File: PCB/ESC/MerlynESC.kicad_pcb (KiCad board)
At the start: 4 copper layers, 30.5 x 31.9 mm, 155 parts, among them M1 BLDC Motor, M2 BLDC Motor, M3 BLDC Motor, M4 BLDC Motor, Q1 JMSL0302AU, Q10 JMSL0302AU, Q11 JMSL0302AU, Q12 JMSL0302AU, Q13 JMSL0302AU, Q14 JMSL0302AU, Q15 JMSL0302AU, Q16 JMSL0302AU, Q17 JMSL0302AU, Q18 JMSL0302AU, Q19 JMSL0302AU, Q2 JMSL0302AU, Q20 JMSL0302AU, Q21 JMSL0302AU, Q22 JMSL0302AU, Q23 JMSL0302AU, Q24 JMSL0302AU, Q3 JMSL0302AU, Q4 JMSL0302AU, Q5 JMSL0302AU, Q6 JMSL0302AU, Q7 JMSL0302AU, Q8 JMSL0302AU, Q9 JMSL0302AU, U1 HT75C0-1, U10 EG6288, U11 EFM8BB21F16G, U2 HT7533-1, U3 EFM8BB21F16G, U4 EG6288, U5 EG6288, U6 EFM8BB21F16G, U7 INA139NA, U8 EG6288, U9 EFM8BB21F16G

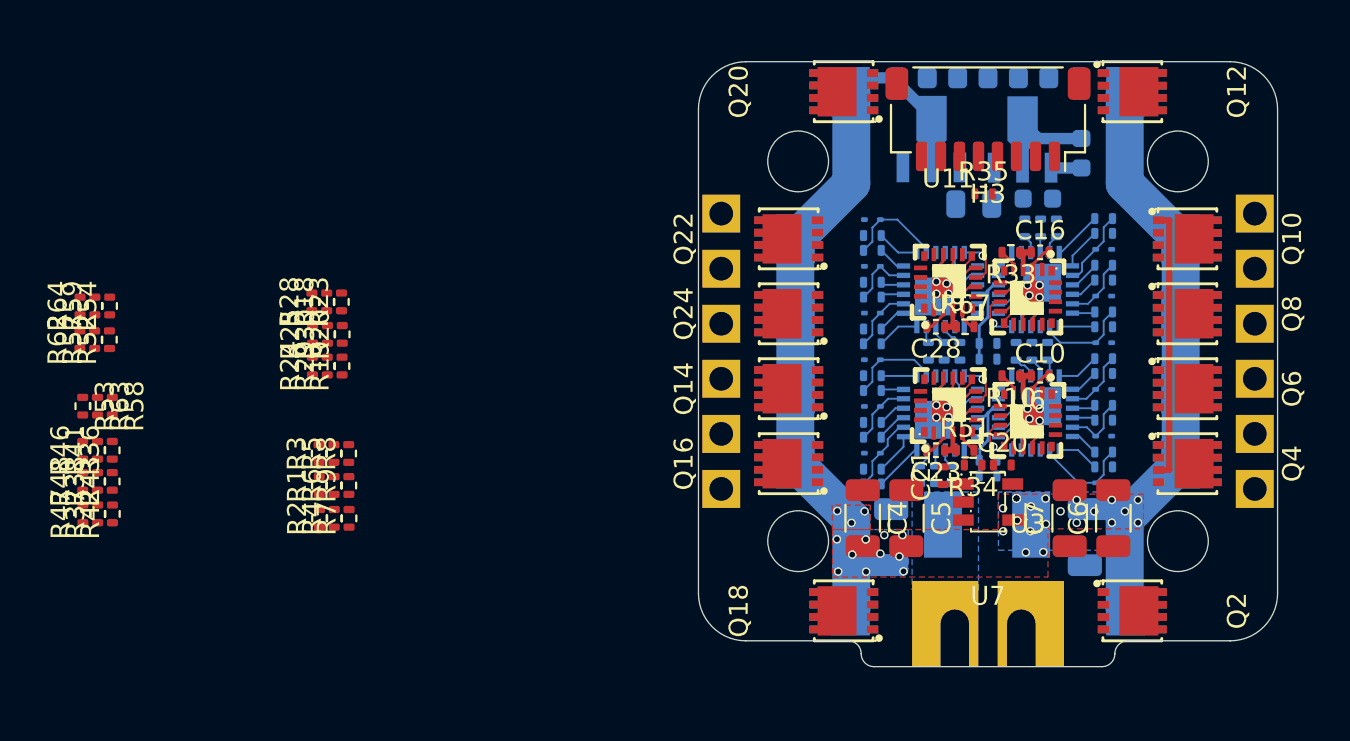
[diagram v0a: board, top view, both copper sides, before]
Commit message: checkpoint
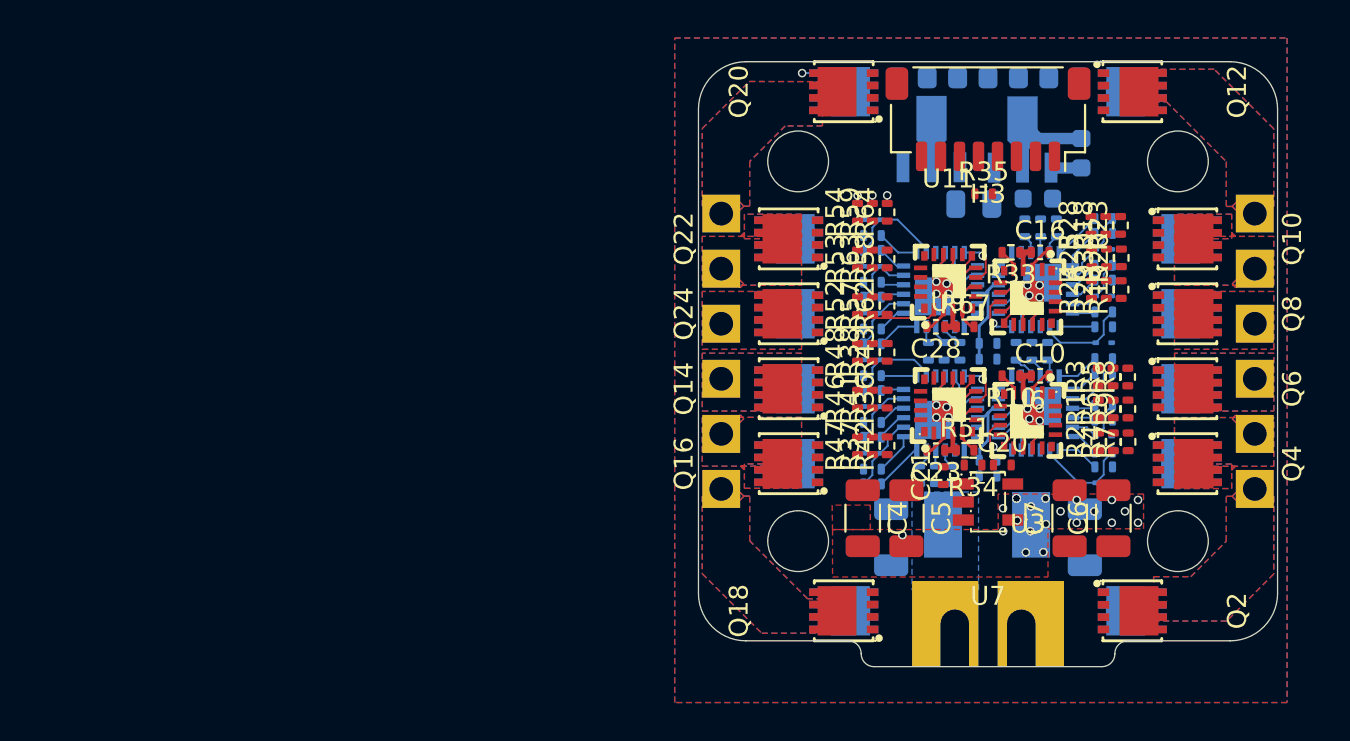
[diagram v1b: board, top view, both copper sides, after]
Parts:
- moved R64 42.8 mm to (150.1, 94.6)
- moved R62 42.6 mm to (150.1, 99.5)
- moved R53 41.5 mm to (148.6, 97.1), turned to 90 degrees
- moved R58 41.5 mm to (150.1, 97.1), turned to 90 degrees
- moved R63 41.5 mm to (149.3, 97.1), turned to 90 degrees
- moved R38 41.4 mm to (149.3, 102.0)
- moved R43 41.4 mm to (150.1, 102.0)
- moved R48 41.4 mm to (148.6, 102.0)
- moved R59 41.2 mm to (149.3, 94.6)
- moved R1 41.2 mm to (161.2, 105.0)
- moved R6 41.2 mm to (162.0, 105.0)
- moved R9 41.2 mm to (162.8, 105.0)
- moved R18 41.2 mm to (161.6, 95.3)
- moved R19 41.2 mm to (162.4, 98.7)
- moved R2 41.2 mm to (161.2, 106.7)
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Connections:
- U11 pad 1: M4_BEMF3 -> M4_BEMF1
- U11 pad 19: M4_BEMFCommon -> M4_BEMF3
- U11 pad 2: M4_BEMF2 -> M4_BEMFCommon
- U11 pad 20: M4_BEMF1 -> M4_BEMF2
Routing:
- net +BATT: track 71.2 -> 3.40 mm, vias 34 -> 22
- net GND: track 27.8 -> 13.5 mm
- net M4_PHASE3: track 0.00 -> 13.3 mm, vias 0 -> 1
- net M4_PHASE2: track 0.00 -> 10.1 mm, vias 0 -> 1
- net M4_PHASE1: track 0.00 -> 7.98 mm, vias 0 -> 1
- net M4_BEMFCommon: track 0.00 -> 4.37 mm
- net Net-(Q19-G): track 0.00 -> 0.67 mm, vias 0 -> 1
- added copper zone on F.Cu, net GND
- added copper zone on B.Cu, net M1_PHASE1
- added copper zone on F.Cu, net M1_PHASE1
- added copper zone on B.Cu, net M1_PHASE2
- added copper zone on F.Cu, net M1_PHASE2
- added copper zone on B.Cu, net M1_PHASE3
- added copper zone on F.Cu, net M1_PHASE3
- added copper zone on B.Cu, net M2_PHASE1
- added copper zone on F.Cu, net M2_PHASE1
- added copper zone on B.Cu, net M2_PHASE2
- added copper zone on F.Cu, net M2_PHASE2
- added copper zone on B.Cu, net M2_PHASE3
- added copper zone on F.Cu, net M2_PHASE3
- added copper zone on B.Cu, net M3_PHASE1
- added copper zone on F.Cu, net M3_PHASE1
- added copper zone on B.Cu, net M3_PHASE2
- added copper zone on F.Cu, net M3_PHASE2
- added copper zone on B.Cu, net M3_PHASE3
- added copper zone on F.Cu, net M3_PHASE3
- added copper zone on B.Cu, net M4_PHASE1
- added copper zone on F.Cu, net M4_PHASE1
- added copper zone on B.Cu, net M4_PHASE2
- added copper zone on F.Cu, net M4_PHASE2
- added copper zone on B.Cu, net M4_PHASE3
- added copper zone on F.Cu, net M4_PHASE3
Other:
- copper layers 4 -> 6

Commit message: checkpoint
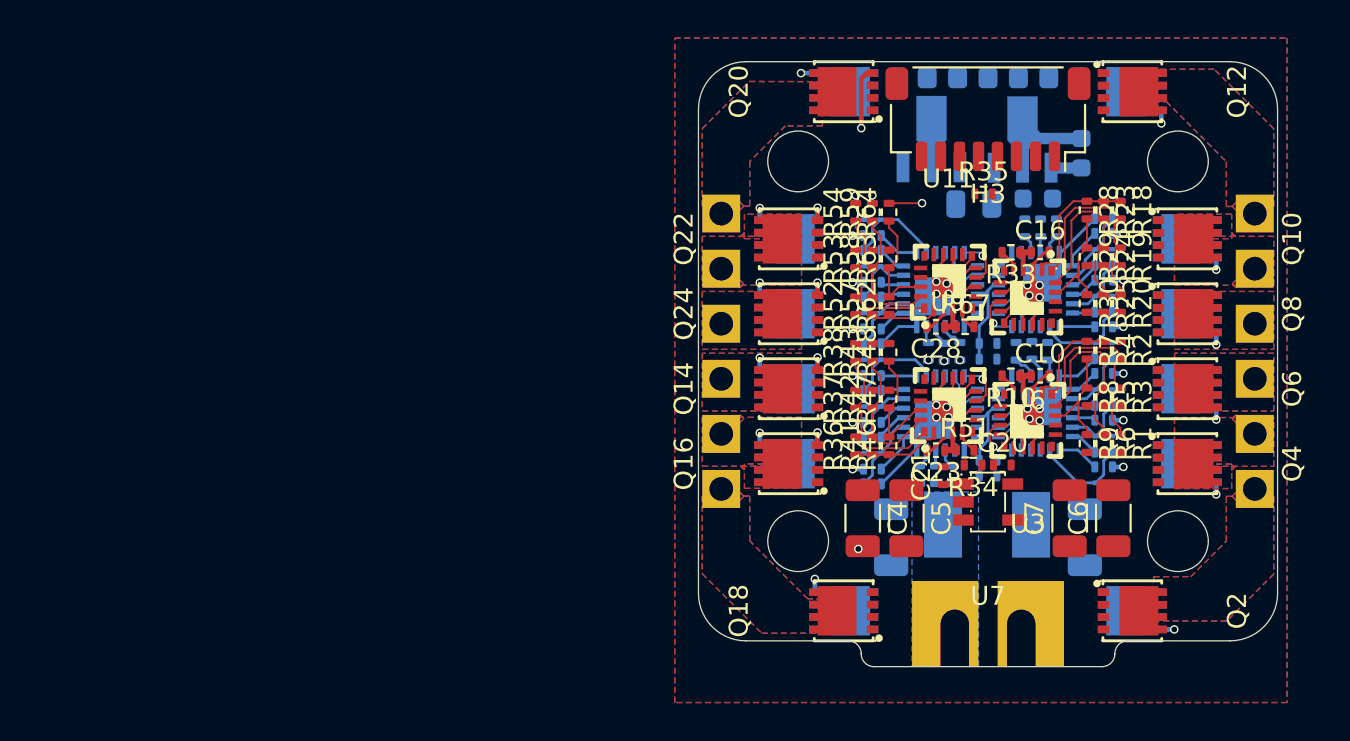
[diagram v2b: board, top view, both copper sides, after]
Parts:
- moved R7 5.29 mm to (160.6, 101.9), turned to -90 degrees
- moved R2 4.96 mm to (162.4, 101.9), turned to -90 degrees
- moved R4 4.86 mm to (161.5, 101.9), turned to -90 degrees
- moved R36 2.97 mm to (148.5, 106.9)
- moved R46 2.97 mm to (150.2, 106.9)
- moved R47 2.97 mm to (150.2, 104.5)
- moved R9 2.82 mm to (160.6, 106.8), turned to -90 degrees
- moved R30 2.61 mm to (160.6, 99.4), turned to -90 degrees
- moved R37 2.61 mm to (148.5, 104.5)
- moved R42 2.58 mm to (149.3, 104.5)
- moved R25 2.48 mm to (161.5, 99.4), turned to -90 degrees
- moved R41 2.46 mm to (149.3, 106.9)
- moved R20 2.40 mm to (162.4, 99.4), turned to -90 degrees
- moved R8 2.39 mm to (160.6, 104.3), turned to -90 degrees
- moved R1 2.16 mm to (162.4, 106.8), turned to -90 degrees
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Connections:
- U3 pad 1: M1_BEMF3 -> M1_BEMF1
- U3 pad 19: M1_BEMFCommon -> M1_BEMF3
- U3 pad 2: M1_BEMF2 -> M1_BEMFCommon
- U3 pad 20: M1_BEMF1 -> M1_BEMF2
- U6 pad 1: M2_BEMF3 -> M2_BEMF1
- U6 pad 19: M2_BEMFCommon -> M2_BEMF3
- U6 pad 2: M2_BEMF2 -> M2_BEMFCommon
- U6 pad 20: M2_BEMF1 -> M2_BEMF2
- U9 pad 1: M3_BEMF3 -> M3_BEMF1
- U9 pad 19: M3_BEMFCommon -> M3_BEMF3
- U9 pad 2: M3_BEMF2 -> M3_BEMFCommon
- U9 pad 20: M3_BEMF1 -> M3_BEMF2
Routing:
- net Net-(Q20-G): track 0.00 -> 17.0 mm, vias 0 -> 2
- net Net-(Q22-G): track 0.00 -> 13.3 mm, vias 0 -> 2
- net Net-(Q24-G): track 0.00 -> 11.9 mm, vias 0 -> 2
- net M2_BEMF1: track 0.00 -> 11.1 mm
- net Net-(Q1-G): track 0.00 -> 10.9 mm, vias 0 -> 2
- net M1_BEMF1: track 0.00 -> 10.3 mm
- net Net-(Q19-G): track 0.67 -> 11.0 mm, vias 1 -> 2
- net M2_BEMF2: track 0.00 -> 10.0 mm
- net M1_BEMF2: track 0.00 -> 9.26 mm
- net M3_BEMF1: track 0.00 -> 8.82 mm
- net M4_BEMF1: track 0.00 -> 8.48 mm
- net Net-(Q11-G): track 0.00 -> 7.83 mm, vias 0 -> 2
- net Net-(Q17-G): track 0.00 -> 7.82 mm, vias 0 -> 2
- net Net-(Q3-G): track 0.00 -> 7.72 mm, vias 0 -> 2
- net Net-(Q21-G): track 0.00 -> 7.72 mm, vias 0 -> 2
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- added copper zone on In3.Cu, net +BATT
- added copper zone on In4.Cu, net +BATT
- added copper zone on In1.Cu, net GND
- added copper zone on In2.Cu, net GND
- added copper zone on In1.Cu, net M1_PHASE1
- added copper zone on In2.Cu, net M1_PHASE1
- added copper zone on In3.Cu, net M1_PHASE1
- added copper zone on In4.Cu, net M1_PHASE1
- added copper zone on In1.Cu, net M1_PHASE2
- added copper zone on In2.Cu, net M1_PHASE2
- added copper zone on In3.Cu, net M1_PHASE2
- added copper zone on In4.Cu, net M1_PHASE2
- added copper zone on In1.Cu, net M1_PHASE3
- added copper zone on In2.Cu, net M1_PHASE3
- added copper zone on In3.Cu, net M1_PHASE3
- added copper zone on In4.Cu, net M1_PHASE3
- added copper zone on In1.Cu, net M2_PHASE1
- added copper zone on In2.Cu, net M2_PHASE1
- added copper zone on In3.Cu, net M2_PHASE1
- added copper zone on In4.Cu, net M2_PHASE1
- added copper zone on In1.Cu, net M2_PHASE2
- added copper zone on In2.Cu, net M2_PHASE2
- added copper zone on In3.Cu, net M2_PHASE2
- added copper zone on In4.Cu, net M2_PHASE2
- added copper zone on In1.Cu, net M2_PHASE3
- added copper zone on In2.Cu, net M2_PHASE3
- added copper zone on In3.Cu, net M2_PHASE3
- added copper zone on In4.Cu, net M2_PHASE3
- added copper zone on In1.Cu, net M3_PHASE1
- added copper zone on In2.Cu, net M3_PHASE1
- added copper zone on In3.Cu, net M3_PHASE1
- added copper zone on In4.Cu, net M3_PHASE1
- added copper zone on In1.Cu, net M3_PHASE2
- added copper zone on In2.Cu, net M3_PHASE2
- added copper zone on In3.Cu, net M3_PHASE2
- added copper zone on In4.Cu, net M3_PHASE2
- added copper zone on In1.Cu, net M3_PHASE3
- added copper zone on In2.Cu, net M3_PHASE3
- added copper zone on In3.Cu, net M3_PHASE3
- added copper zone on In4.Cu, net M3_PHASE3
- added copper zone on In1.Cu, net M4_PHASE1
- added copper zone on In2.Cu, net M4_PHASE1
- added copper zone on In3.Cu, net M4_PHASE1
- added copper zone on In4.Cu, net M4_PHASE1
- added copper zone on In1.Cu, net M4_PHASE2
- added copper zone on In2.Cu, net M4_PHASE2
- added copper zone on In3.Cu, net M4_PHASE2
- added copper zone on In4.Cu, net M4_PHASE2
- added copper zone on In1.Cu, net M4_PHASE3
- added copper zone on In2.Cu, net M4_PHASE3
- added copper zone on In3.Cu, net M4_PHASE3
- added copper zone on In4.Cu, net M4_PHASE3
- added copper zone on In3.Cu, net Net-(BT1-+)
- added copper zone on In4.Cu, net Net-(BT1-+)
- removed copper zone on F.Cu, net +BATT

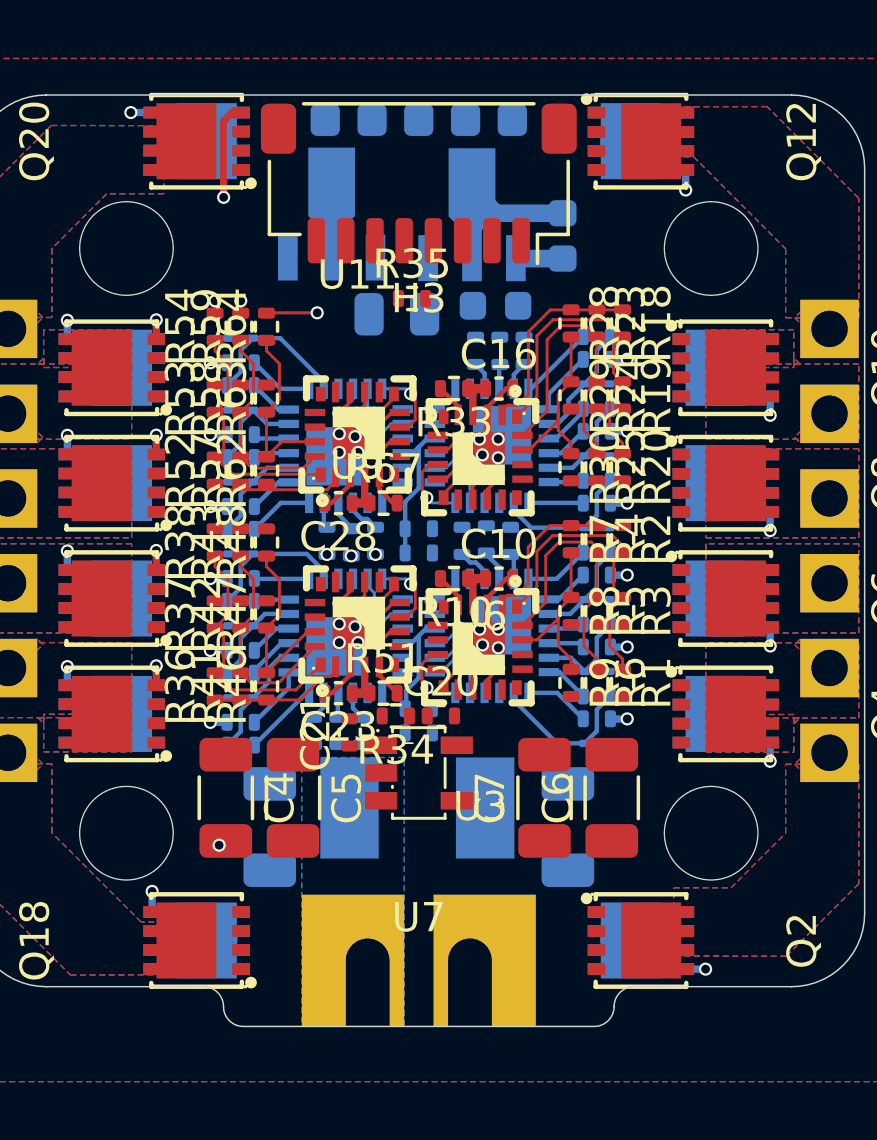
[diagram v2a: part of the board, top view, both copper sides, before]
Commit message: checkpoint
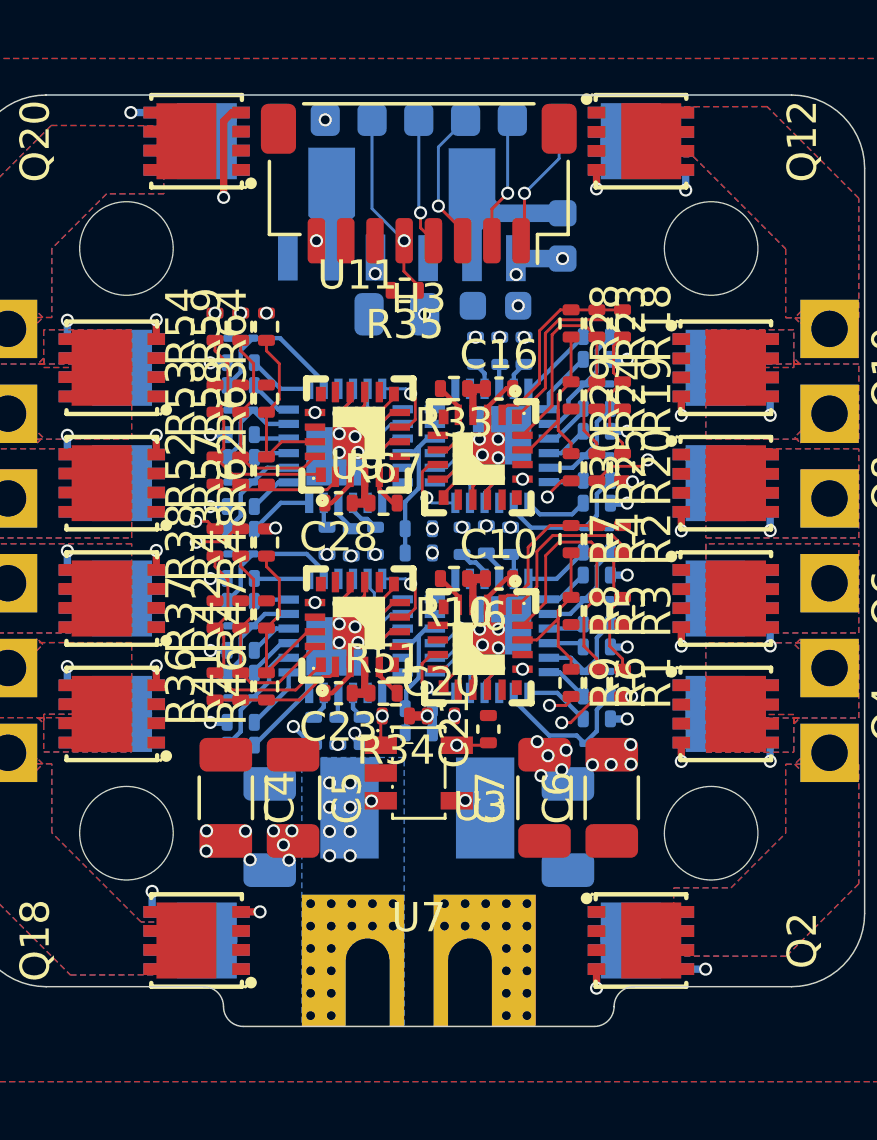
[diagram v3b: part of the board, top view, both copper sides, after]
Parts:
- moved C21 4.74 mm to (157.8, 108.4)
- moved R35 0.38 mm to (154.9, 93.4), turned to 180 degrees
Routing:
- net M3_DSHOT: track 0.00 -> 23.1 mm, vias 0 -> 2
- net M1_DSHOT: track 0.00 -> 22.8 mm, vias 0 -> 2
- net Net-(Q2-G): track 0.00 -> 18.2 mm, vias 0 -> 2
- net M4_DSHOT: track 0.00 -> 18.0 mm, vias 0 -> 2
- net M2_DSHOT: track 0.00 -> 15.4 mm, vias 0 -> 2
- net M3_PHASE3: track 2.01 -> 17.2 mm, vias 0 -> 1
- net M2_PHASE3: track 0.00 -> 14.8 mm, vias 0 -> 1
- net Net-(Q4-G): track 0.00 -> 12.7 mm, vias 0 -> 2
- net Net-(Q8-G): track 0.00 -> 10.9 mm, vias 0 -> 2
- net Net-(Q6-G): track 0.00 -> 10.7 mm, vias 0 -> 2
- net Net-(Q14-G): track 0.66 -> 10.8 mm, vias 1 -> 2
- net Net-(Q18-G): track 0.00 -> 9.95 mm, vias 0 -> 2
- net Net-(Q10-G): track 0.00 -> 8.36 mm, vias 0 -> 2
- net M1_PHASE2: track 0.00 -> 8.05 mm, vias 0 -> 1
- net Net-(Q12-G): track 0.00 -> 7.64 mm, vias 0 -> 2
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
